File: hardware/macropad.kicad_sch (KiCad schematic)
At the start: 27 parts, among them J2 Conn_01x06, J3 I2C Screen, J4 SPI Screen, SW1 SW_Push, SW10 SW_Push, SW2 SW_Push, SW3 SW_Push, SW4 SW_Push, SW5 SW_Push, SW6 SW_Push, SW7 SW_Push, SW8 SW_Push, SW9 SW_Push, U1 Pico

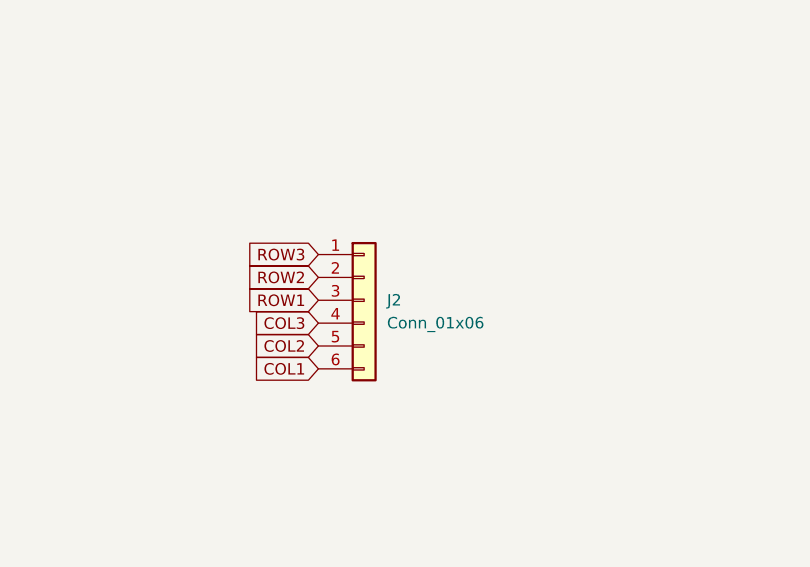
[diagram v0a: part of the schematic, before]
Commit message: :construction: Some routing
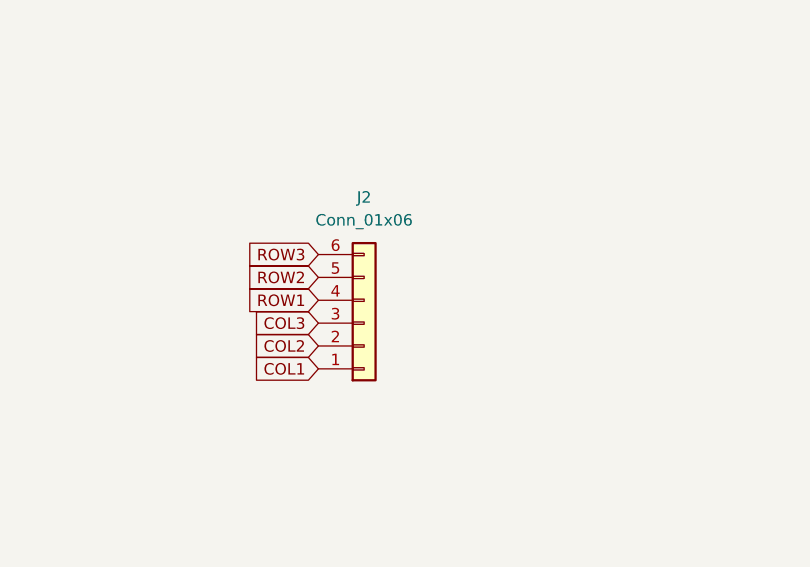
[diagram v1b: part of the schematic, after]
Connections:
- net COL1: now also J2.1 (Pin_1); no longer J2.6 (Pin_6)
- net COL2: now also J2.2 (Pin_2); no longer J2.5 (Pin_5)
- net COL3: now also J2.3 (Pin_3); no longer J2.4 (Pin_4)
- net ROW1: now also J2.4 (Pin_4); no longer J2.3 (Pin_3)
- net ROW2: now also J2.5 (Pin_5); no longer J2.2 (Pin_2)
- net ROW3: now also J2.6 (Pin_6); no longer J2.1 (Pin_1)
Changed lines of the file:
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@@
     (pin "2")
   )
-  (symbol (lib_id "Connector_Generic:Conn_01x06") (at 102.87 142.24 0) (unit 1)
+  (symbol (lib_id "Connector_Generic:Conn_01x06") (at 102.87 144.78 0) (mirror x) (unit 1)
     (in_bom yes) (on_board yes) (fields_autoplaced)
-    (property "Reference" "J2" (id 0) (at 105.41 142.2399 0)
-      (effects (font (size 1.27 1.27)) (justify left))
-    )
-    (property "Value" "Conn_01x06" (id 1) (at 105.41 144.7799 0)
-      (effects (font (size 1.27 1.27)) (justify left))
-    )
-    (property "Footprint" "Connector_PinHeader_2.54mm:PinHeader_1x06_P2.54mm_Vertical" (id 2) (at 102.87 142.24 0)
+    (property "Reference" "J2" (id 0) (at 102.87 130.81 0))
+    (property "Value" "Conn_01x06" (id 1) (at 102.87 133.35 0))
+    (property "Footprint" "Connector_PinHeader_2.54mm:PinHeader_1x06_P2.54mm_Vertical" (id 2) (at 102.87 144.78 0)
       (effects (font (size 1.27 1.27)) hide)
     )
-    (property "Datasheet" "~" (id 3) (at 102.87 142.24 0)
+    (property "Datasheet" "~" (id 3) (at 102.87 144.78 0)
       (effects (font (size 1.27 1.27)) hide)
     )
